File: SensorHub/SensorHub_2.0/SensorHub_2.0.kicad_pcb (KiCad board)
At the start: 4 copper layers, 30 x 28 mm, 67 parts, among them J2 658561423020, J3 658561423020, J5 FTSH-105-01-L-DV-K-A, J6 USB_C_Receptacle_USB2.0_16P, J8 USB_C_Receptacle_USB2.0_16P, SW1 SW_Push, SW2 SW_Push, U1 R7FA4E2B93CFM#AA0, U10 LMV339, U2 MYRGM080200C41RA, U3 TCAN334, U4 USBLC6-4SC6, U5 TMUX154EDGS, U6 LSM6DSM, U7 USBLC6-4SC6, Y1 ASH7KW-32.768KHZ-L-T

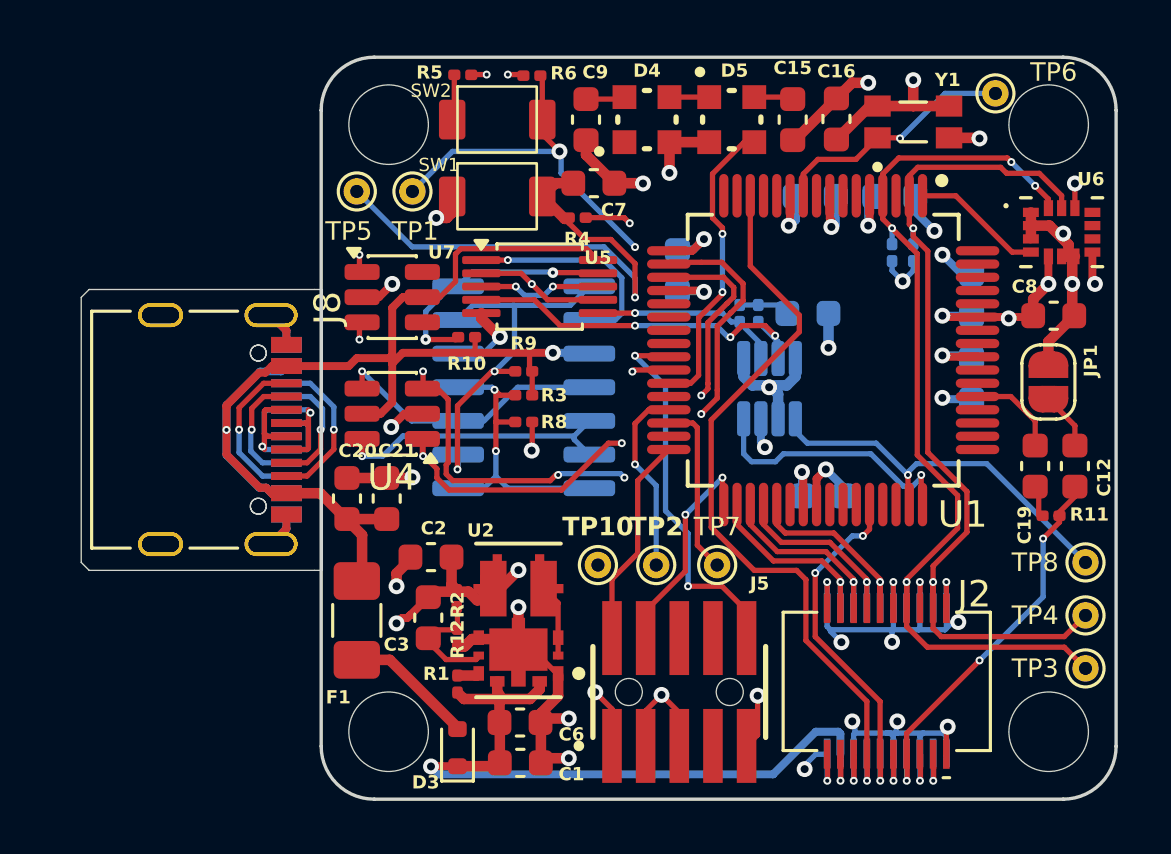
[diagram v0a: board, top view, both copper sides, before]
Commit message: PCB fix
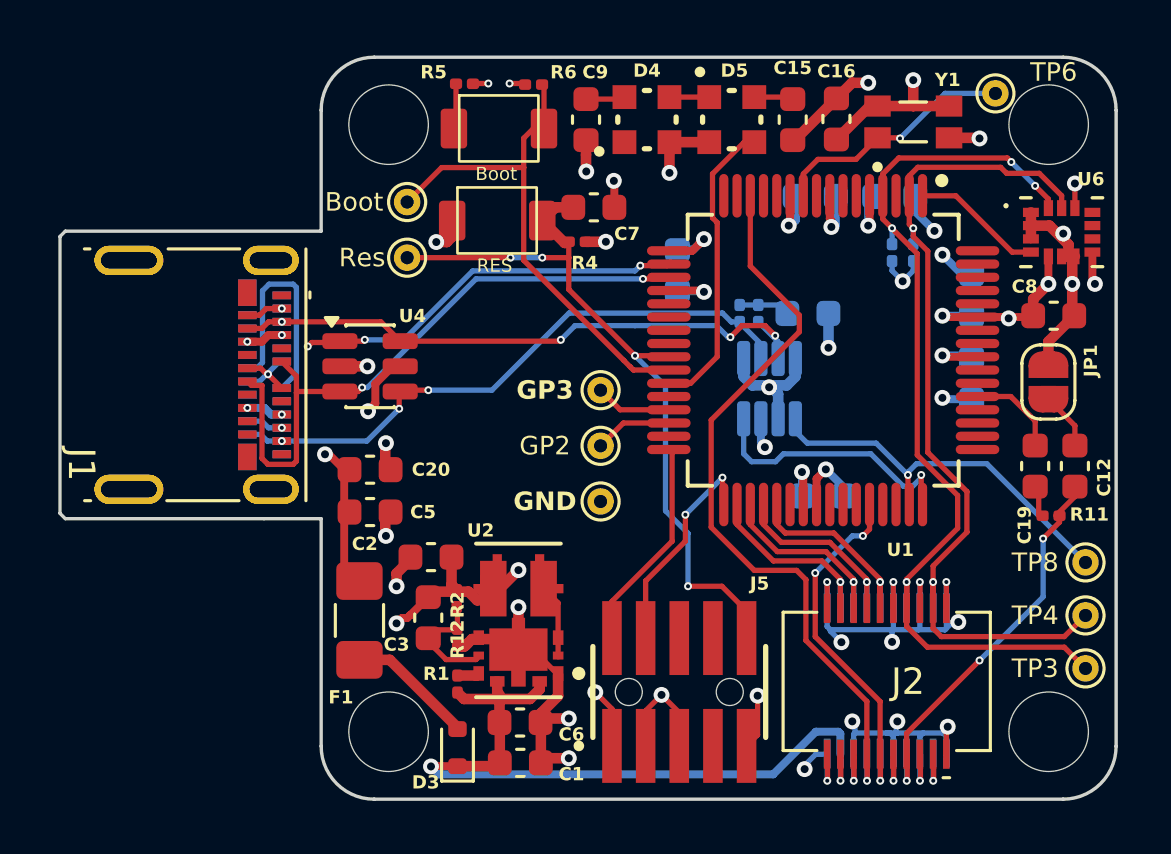
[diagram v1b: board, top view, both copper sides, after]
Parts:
- removed C21: 0.1 uF, Capacitor_SMD:C_0603_1608Metric
- removed FRAME1: FRAME-LEDGER, SensorHub MicroMod Carrier v1.1.0b:CREATIVE_COMMONS
- removed J6, J8: USB_C_Receptacle_USB2.0_16P, Connector_USB:USB_C_Receptacle_Palconn_UTC16-G
- removed R10, R8, R9: 5.1 K, Resistor_SMD:R_0201_0603Metric
- removed R3: 100 K, Resistor_SMD:R_0201_0603Metric
- removed U10: LMV339, Package_SO:SOIC-14_3.9x8.7mm_P1.27mm
- removed U5: TMUX154EDGS, Package_SO:VSSOP-10_3x3mm_P0.5mm
- removed U7: USBLC6-4SC6, Package_TO_SOT_SMD:SOT-23-6
- added C5: 0.1 uF, Capacitor_SMD:C_0603_1608Metric, F.Cu at (140.0, 88.0)
- added J1: USB_C_Receptacle, Connector_USB:USB_C_Receptacle_Molex_105450-0101, F.Cu at (133.5, 82.8)
- added J4: USB_C_Receptacle, Connector_USB:USB_C_Receptacle_Molex_105450-0101, B.Cu at (133.5, 82.8)
- moved GP3 6.93 mm to (148.7, 83.4)
- moved GP2 6.29 mm to (148.7, 85.5)
- moved Res 3.14 mm to (141.4, 78.4)
- moved GND 2.40 mm to (148.7, 87.6)
- moved U4 1.98 mm to (140.0, 82.5), turned to 0 degrees
- moved C20 1.39 mm to (140.0, 86.4), turned to 0 degrees
- moved C7 0.91 mm to (148.4, 76.5)
- moved R4 0.91 mm to (147.8, 77.8)
- moved RES 0.91 mm to (144.8, 77.0)
- moved Boot 0.45 mm to (141.4, 76.3)
- moved Boot 0.34 mm to (144.9, 73.5)
- moved R5 0.34 mm to (143.6, 71.8)
- moved R6 0.34 mm to (146.2, 71.9)
- moved F1 0.10 mm to (139.6, 92.1)
- turned U$40 to 90 degrees
- renumbered SW2 to Boot, TP1 to Boot, TP10 to GND, TP7 to GP2, TP2 to GP3, SW1 to RES, TP5 to Res
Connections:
- J2 pad 2: +3.3V -> /+3.3V
- J3 pad 12: +3.3V -> /+3.3V
- U4 pad 1: /USB_DP -> /USB_DM
- U4 pad 3: /USB_DM -> /USB_DP
- U4 pad 4: /USB_C_2.0+SBUS/CC2 -> /Can_L
- U4 pad 6: /USB_C_2.0+SBUS/CC1 -> /Can_H
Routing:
- net /V_Bus: track 50.3 -> 18.5 mm, vias 2 -> 6
- net /USB_C_2.0+SBUS/SBU2: track 26.3 -> 0.00 mm, vias 4 -> 0
- net /USB_C_2.0+SBUS/SBU1: track 22.8 -> 0.00 mm, vias 3 -> 0
- net /USB_C_2.0+SBUS/CC1: track 20.6 -> 0.00 mm, vias 2 -> 0
- net /USB_C_2.0+SBUS/CC2: track 19.1 -> 0.00 mm, vias 2 -> 0
- net /Can_L: track 7.17 -> 24.3 mm, vias 1 -> 4
- net /USB_DM: track 36.4 -> 20.2 mm, vias 5 -> 4
- net Net-(U10D-+): track 13.9 -> 0.00 mm, vias 2 -> 0
- net GND: track 108.0 -> 95.1 mm, vias 42 -> 41
- net Net-(U10B-+): track 11.7 -> 0.00 mm, vias 2 -> 0
- net /Can_H: track 13.7 -> 24.2 mm, vias 3 -> 5
- net /USB_C_2.0+SBUS/EN: track 9.46 -> 0.00 mm, vias 2 -> 0
- net /RES: track 36.9 -> 28.6 mm, vias 3 -> 4
- net /USB_C_2.0+SBUS/cable_orient: track 8.25 -> 0.00 mm, vias 1 -> 0
- net /GP3: track 7.16 -> 2.88 mm, vias 1 -> 0
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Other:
- board text added: "Made on Earth"
- board text added: "RobotPatient.com"
- board text added: "SensorHub_2.0"
